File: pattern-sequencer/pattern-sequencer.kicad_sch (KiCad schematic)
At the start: 59 parts, among them J1 Power, J10 Conn_01x03_Socket, J11 Conn_01x03_Socket, J12 Conn_01x03_Socket, J13 Conn_01x03_Socket, J14 Conn_01x03_Socket, J2 Power, J3 Power, J4 External Clock, J5 Conn_01x03_Socket, J6 Out 1, J7 Out 2, J8 Out 3, J9 Out 4, SW1 IN 1, SW2 IN 2, SW3 IN 3, SW4 IN 4, SW5 CLEAR, SW6 External Clock Select

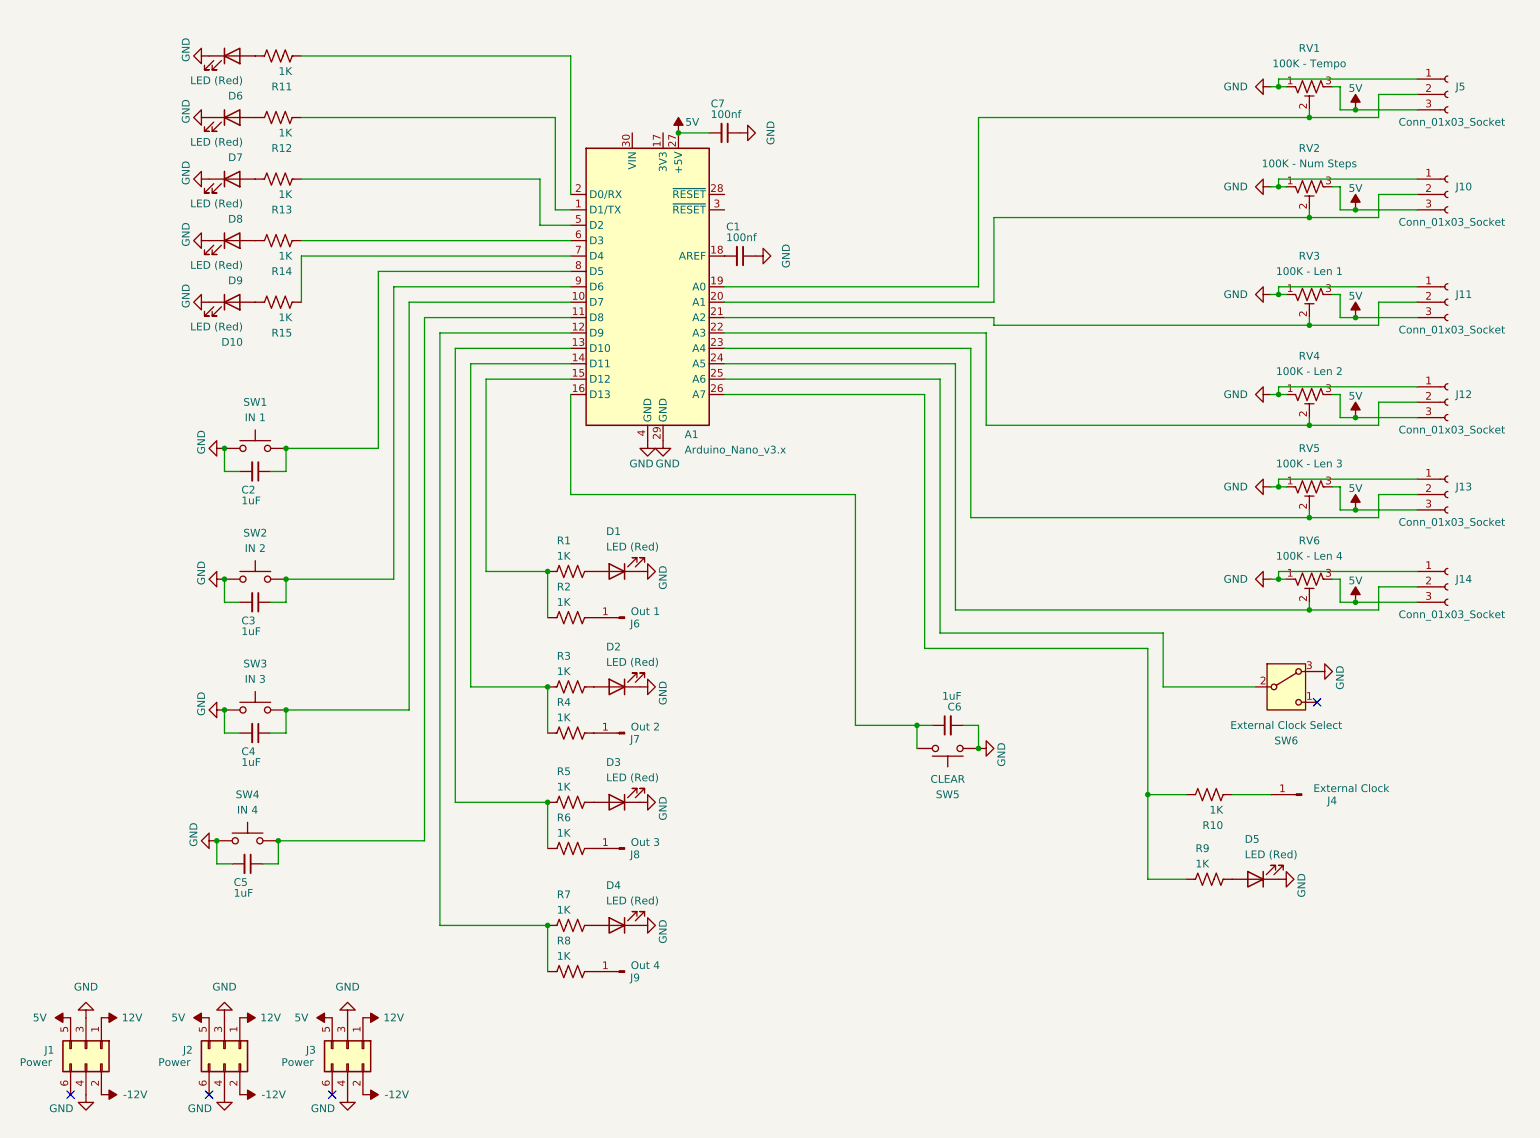
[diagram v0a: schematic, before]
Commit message: Update pattern sequencer
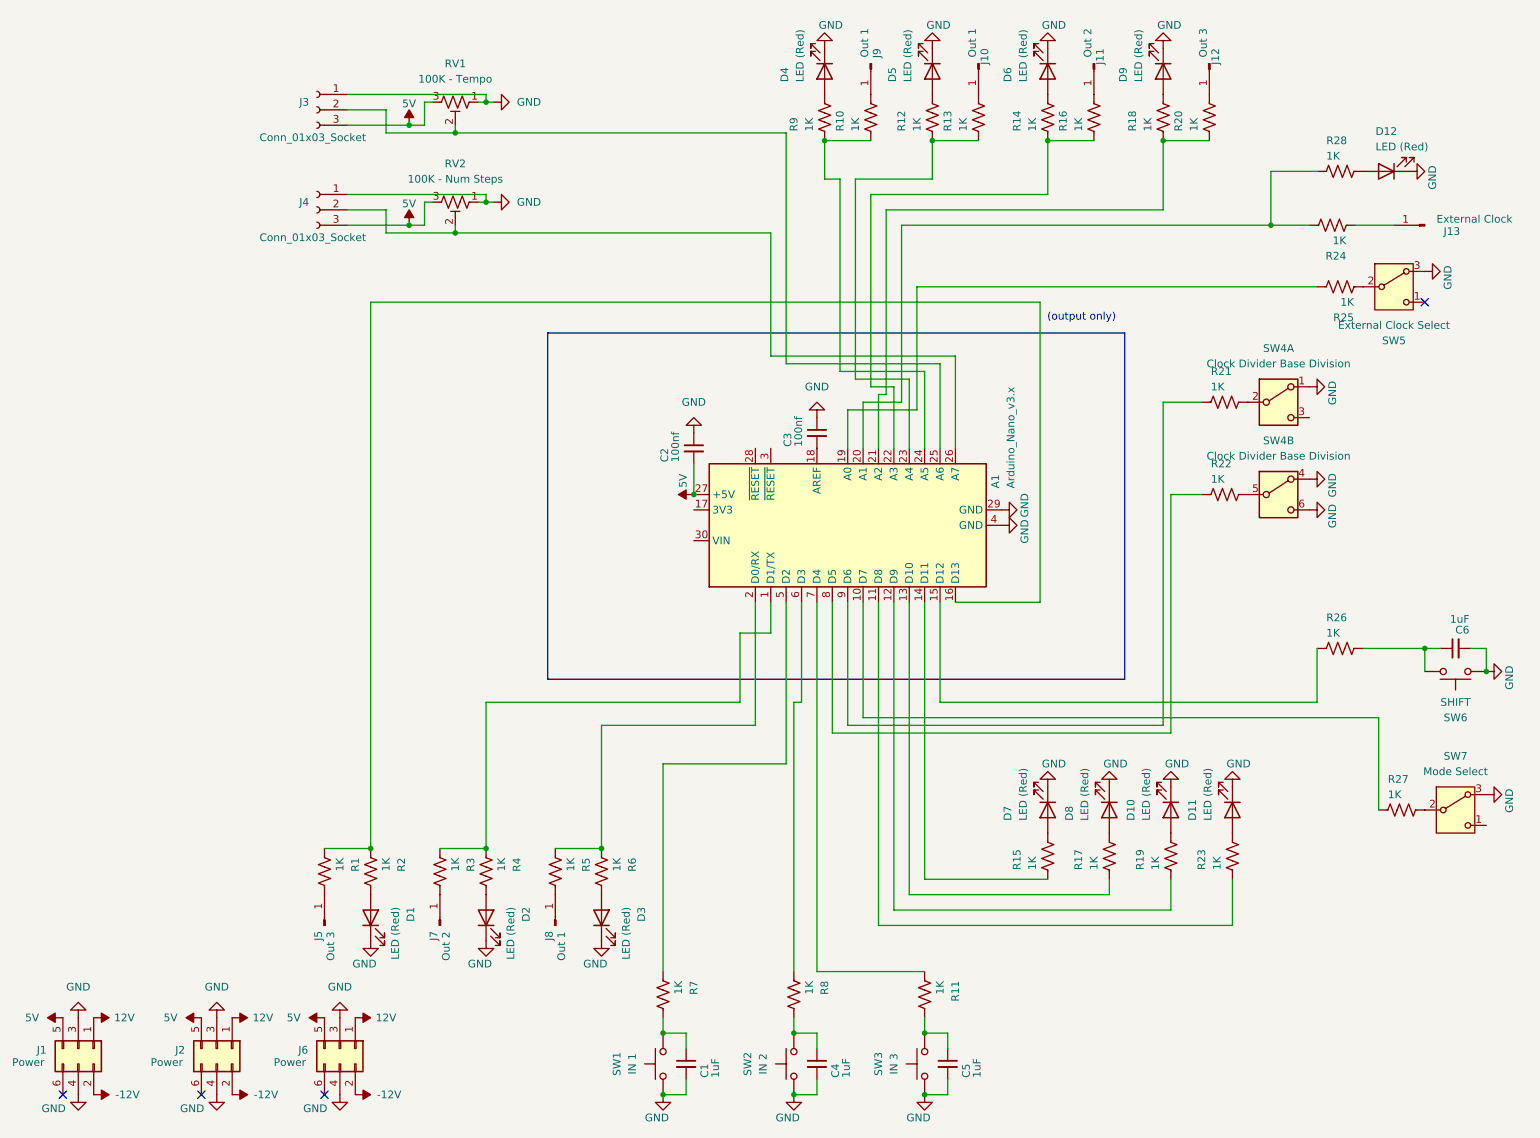
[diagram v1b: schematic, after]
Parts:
- removed C5: 1uF, Capacitor_THT:C_Disc_D4.3mm_W1.9mm_P5.00mm, symbol Device:C_Small
- removed D10: LED (Red), LED_THT:LED_D5.0mm, symbol Device:LED
- removed J11, J12, J13, J14: Conn_01x03_Socket, modular2:pot, symbol Connector:Conn_01x03_Socket
- removed R15: 1K, Resistor_THT:R_Axial_DIN0207_L6.3mm_D2.5mm_P10.16mm_Horizontal, symbol Device:R_US
- removed RV3: 100K - Len 1, modular2:pot-socket, symbol Device:R_Potentiometer_Trim_US
- removed RV4: 100K - Len 2, modular2:pot-socket, symbol Device:R_Potentiometer_Trim_US
- removed RV5: 100K - Len 3, modular2:pot-socket, symbol Device:R_Potentiometer_Trim_US
- removed RV6: 100K - Len 4, modular2:pot-socket, symbol Device:R_Potentiometer_Trim_US
- removed SW4: IN 4, Button_Switch_Keyboard:SW_Cherry_MX_1.00u_PCB, symbol Switch:SW_Push
- added D12, D6, D9: LED (Red), LED_THT:LED_D5.0mm, symbol Device:LED
- added J10: Out 1, modular2:banana-jack, symbol Connector:Conn_01x01_Pin
- added J11: Out 2, modular2:banana-jack, symbol Connector:Conn_01x01_Pin
- added J12: Out 3, modular2:banana-jack, symbol Connector:Conn_01x01_Pin
- added R10, R11, R12, R13, R14, R16, R18, R20, R21, R22, R25, R26, R27, R28: 1K, Resistor_THT:R_Axial_DIN0207_L6.3mm_D2.5mm_P10.16mm_Horizontal, symbol Device:R_US
- added SW4: Clock Divider Base Division, modular2:switch2, symbol Switch:SW_DPDT_x2
- added SW7: Mode Select, modular2:switch1, symbol Switch:SW_Nidec_CAS-120A1
- J9: value Out 4 -> Out 1
- SW6: renamed from SW5; value CLEAR -> SHIFT
- renumbered C2 to C1, C7 to C2, C1 to C3, C3 to C4, C4 to C5, D3 to D1, D7 to D10, D6 to D11, D1 to D3, D9 to D7, J4 to J13, J5 to J3, J10 to J4, J8 to J5, J3 to J6, J6 to J8, R6 to R1, R14 to R15, R13 to R17, R12 to R19, R5 to R2, R11 to R23, R10 to R24, R4 to R3, R3 to R4, R2 to R5, R1 to R6, SW6 to SW5
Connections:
- net GND: now also D12.1 (K), D6.1 (K), D9.1 (K), SW4.1 (A), SW4.4 (A), SW4.6 (C), SW7.3 (A)
- net at R23.2: now also A1.11 (D8); no longer A1.2 (D0/RX)
- net at A1.24 (A5): now also R9.2, R10.2
- net at R1.2, R2.2: now also A1.16 (D13); no longer A1.13 (D10)
- net at A1.6 (D3): now also R8.2; no longer R15.2
- net at R9.1: now also D4.2 (A); no longer D5.2 (A)
- net at R5.2, R6.2: now also A1.2 (D0/RX); no longer A1.15 (D12)
- net at R17.2: now also A1.13 (D10); no longer A1.5 (D2)
- net at J3.2 (Pin_2), RV1.2: now also A1.25 (A6); no longer A1.19 (A0)
- net at A1.23 (A4): now also R12.2, R13.2
- net at SW5.2 (B): now also R25.2; no longer A1.25 (A6)
- net at R19.2: now also A1.12 (D9); no longer A1.1 (D1/TX)
- net at R8.1: now also C4.1, SW2.2; no longer J9.1 (Pin_1)
- net at C5.1, SW3.2: now also R11.1; no longer A1.10 (D7)
- net at A1.22 (A3): now also R14.2, R16.2
- net at A1.21 (A2): now also R18.2, R20.2
- net at R3.2, R4.2: now also A1.1 (D1/TX); no longer A1.14 (D11)
- net at C6.1, SW6.2: now also R26.1; no longer A1.16 (D13)
- net at J4.2 (Pin_2), RV2.2: now also A1.26 (A7); no longer A1.20 (A1)
- net at A1.7 (D4): now also R11.2
- net at C1.1, SW1.2: now also R7.1; no longer A1.8 (D5)
- new net: D9.2 (A), R18.1
- new net: J11.1 (Pin_1), R16.1
- new net: A1.14 (D11), R15.2
- new net: J9.1 (Pin_1), R10.1
- new net: R22.1, SW4.5 (B)
- new net: R27.1, SW7.2 (B)
- new net: A1.5 (D2), R7.2
- new net: J12.1 (Pin_1), R20.1
- new net: A1.10 (D7), R27.2
- new net: A1.15 (D12), R26.2
- new net: A1.19 (A0), R25.1
- new net: A1.20 (A1), R24.1, R28.2
- new net: A1.8 (D5), R22.2
- new net: A1.9 (D6), R21.2
- new net: R21.1, SW4.2 (B)
- new net: D5.2 (A), R12.1
- new net: J10.1 (Pin_1), R13.1
- new net: D12.2 (A), R28.1
- new net: D6.2 (A), R14.1
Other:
- note added: "(output only)"
- moved on the sheet: A1, C1, C2, C3, C4, C5, C6, D1, D10, D11, D2, D3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
